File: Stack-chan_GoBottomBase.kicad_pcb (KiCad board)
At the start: 2 copper layers, 23 x 27 mm, 15 parts, among them CN1 CON_USB-C-16p, CN2 CON_GROVE, CN3 CON_USB-C-16p, J1 Conn_01x03, J2 Conn_01x03

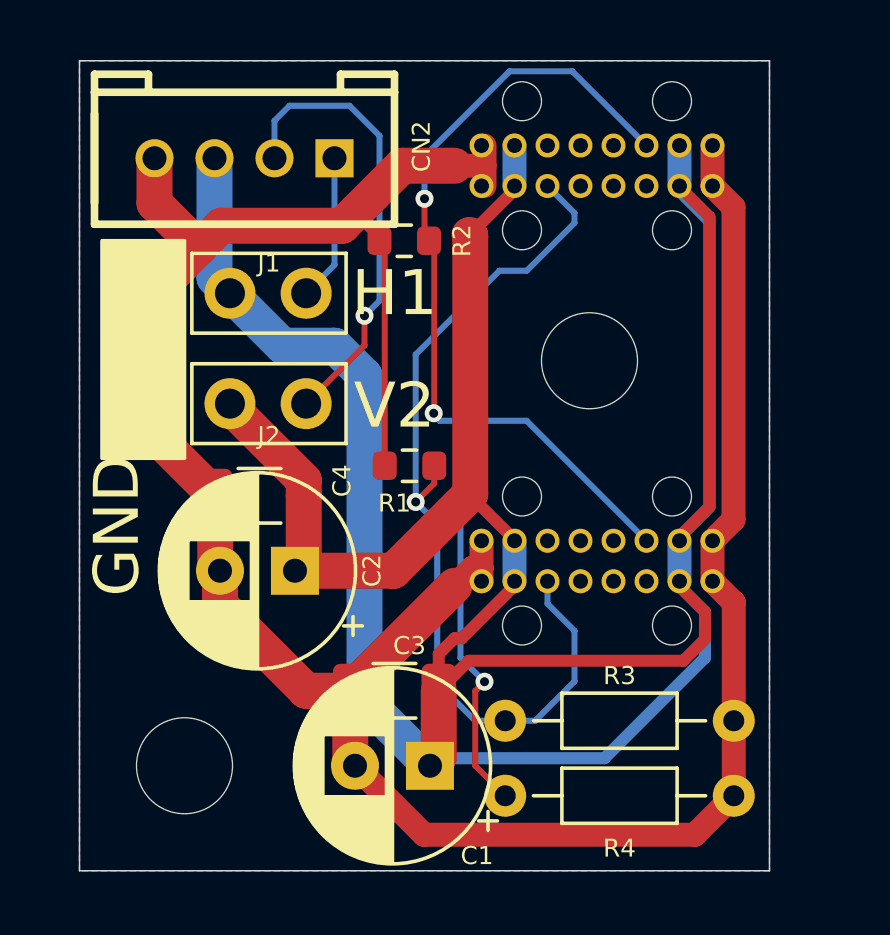
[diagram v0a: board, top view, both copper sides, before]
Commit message: for v1
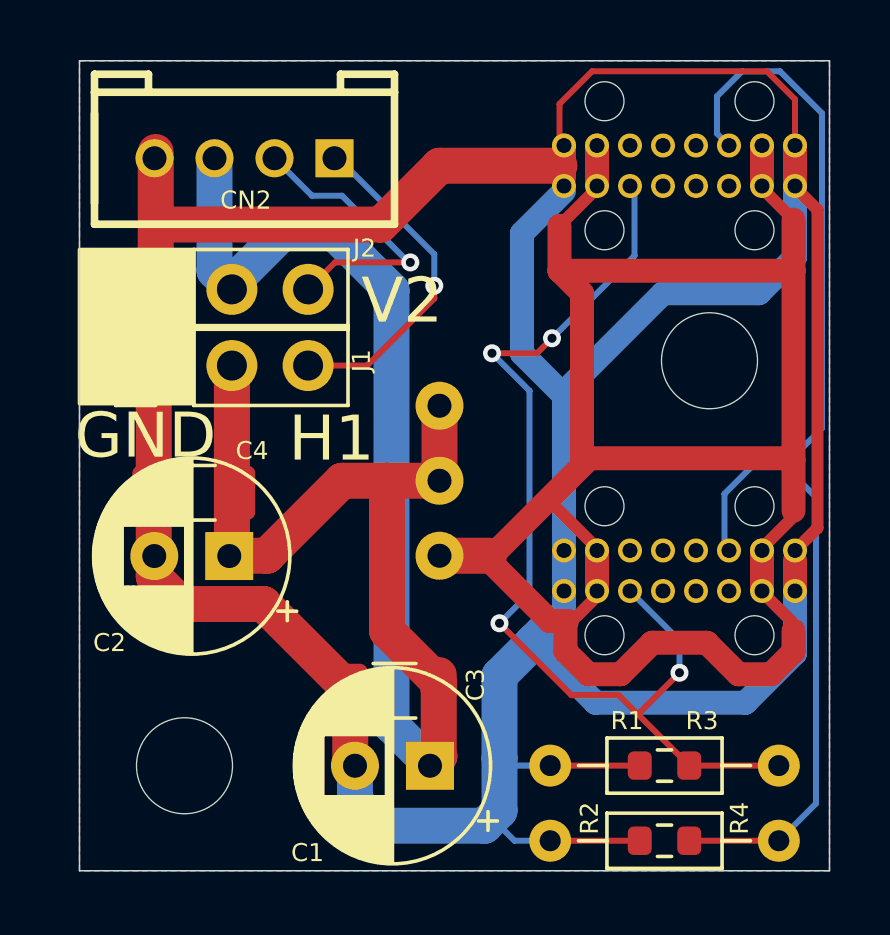
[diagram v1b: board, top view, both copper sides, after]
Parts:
- added SW1: SW_SPDT, akita:SW_SPDT_9x4mm_W2.5mm, B.Cu at (12.0, 14.0)
- moved R2 21.8 mm to (19.5, 26.0)
- moved R1 13.1 mm to (19.5, 23.5)
- moved R4 9.24 mm to (23.3, 26.0), turned to 180 degrees
- moved R3 9.24 mm to (23.3, 23.5), turned to 180 degrees
- moved REF** 4.00 mm to (21.0, 10.0)
- moved J2 3.81 mm to (2.54, 7.62)
- moved CN3 2.77 mm to (20.0, 17.0)
- moved CN1 2.75 mm to (20.0, 3.50)
- moved J1 2.41 mm to (2.54, 10.2)
- moved C2 2.24 mm to (4.99, 16.5)
- moved C4 2.19 mm to (3.81, 14.4)
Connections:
- CN1 pad A4: +5V -> Net-(CN1-PadA4)
- CN1 pad A9: +5V -> Net-(CN1-PadA4)
- CN1 pad B4: +5V -> Net-(CN1-PadA4)
- CN1 pad B9: +5V -> Net-(CN1-PadA4)
- CN3 pad A4: +5V -> Net-(CN1-PadA4)
- CN3 pad A9: +5V -> Net-(CN1-PadA4)
- CN3 pad B4: +5V -> Net-(CN1-PadA4)
- CN3 pad B9: +5V -> Net-(CN1-PadA4)
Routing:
- net Net-(CN1-PadA4): track 0.00 -> 68.6 mm
- net +5V: track 117.7 -> 58.9 mm
- net GND: track 89.6 -> 130.5 mm
- net /SV1: track 4.89 -> 11.3 mm, vias 0 -> 1
- net /SV2: track 15.3 -> 9.75 mm
- net Net-(CN1-PadB5): track 30.8 -> 35.2 mm, vias 1 -> 4
- net Net-(CN1-PadA5): track 40.6 -> 38.8 mm, vias 3 -> 0
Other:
- board size 23 x 27 mm -> 25 x 27 mm
- board text added: "ON"
